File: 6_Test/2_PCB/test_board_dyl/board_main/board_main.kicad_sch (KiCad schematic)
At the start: 26 parts, among them J1 GND_Plane_Jumpers, J2 Analog_Inputs, J3 IOVDD_Jumpers, J4 Digital_Discovery_Output, J5 Power_Input, J6 Clock_Input

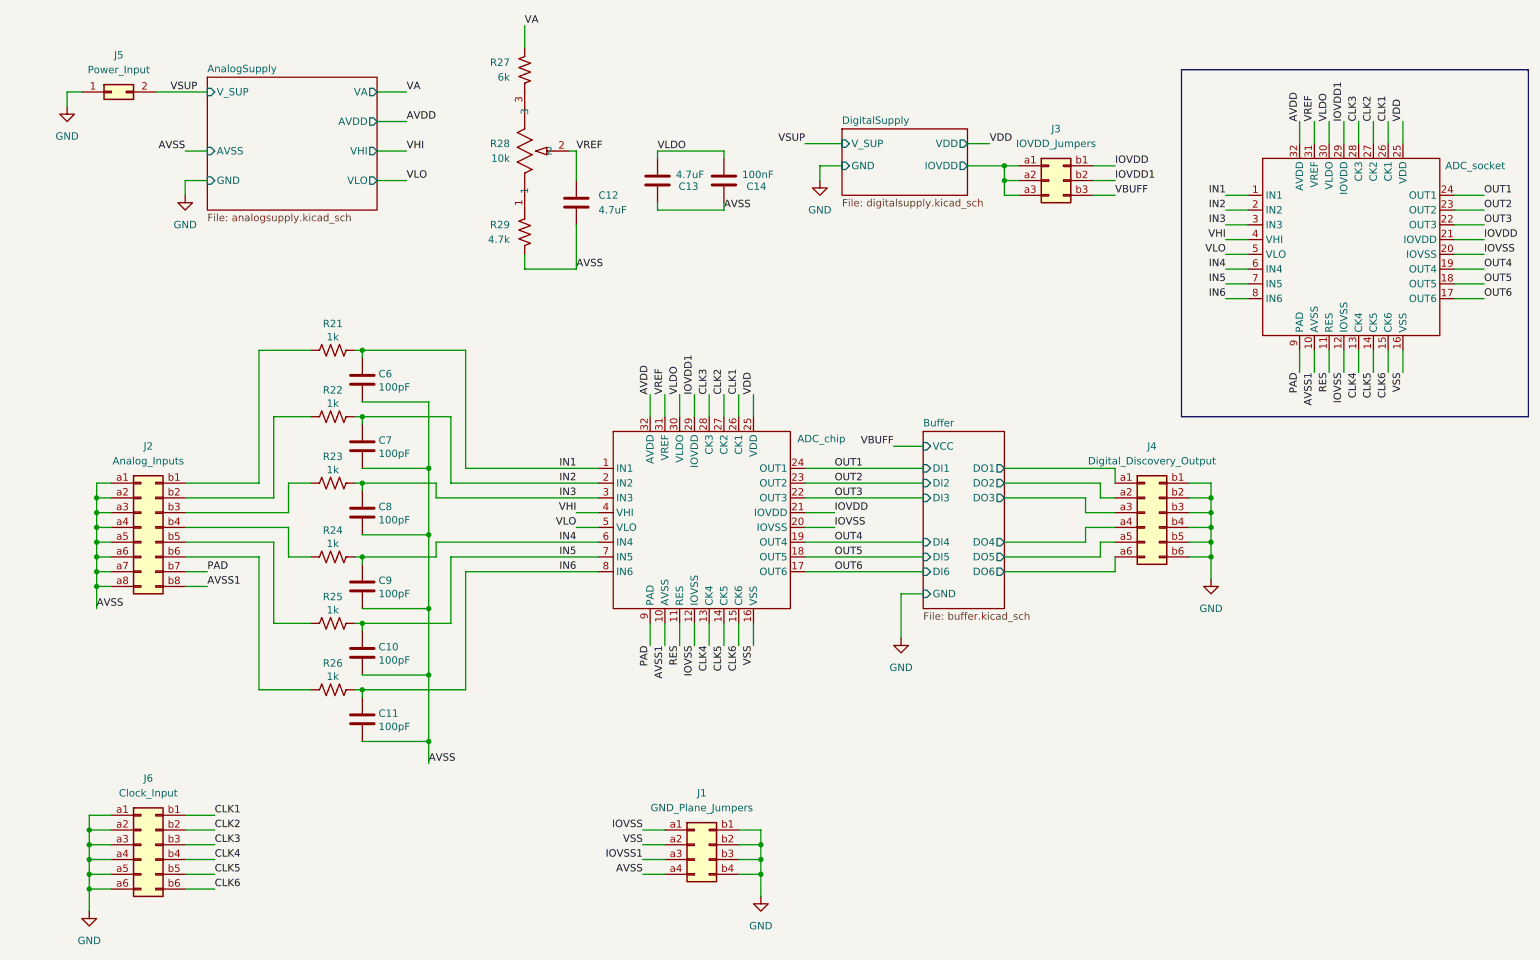
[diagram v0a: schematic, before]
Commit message: Fixed comments
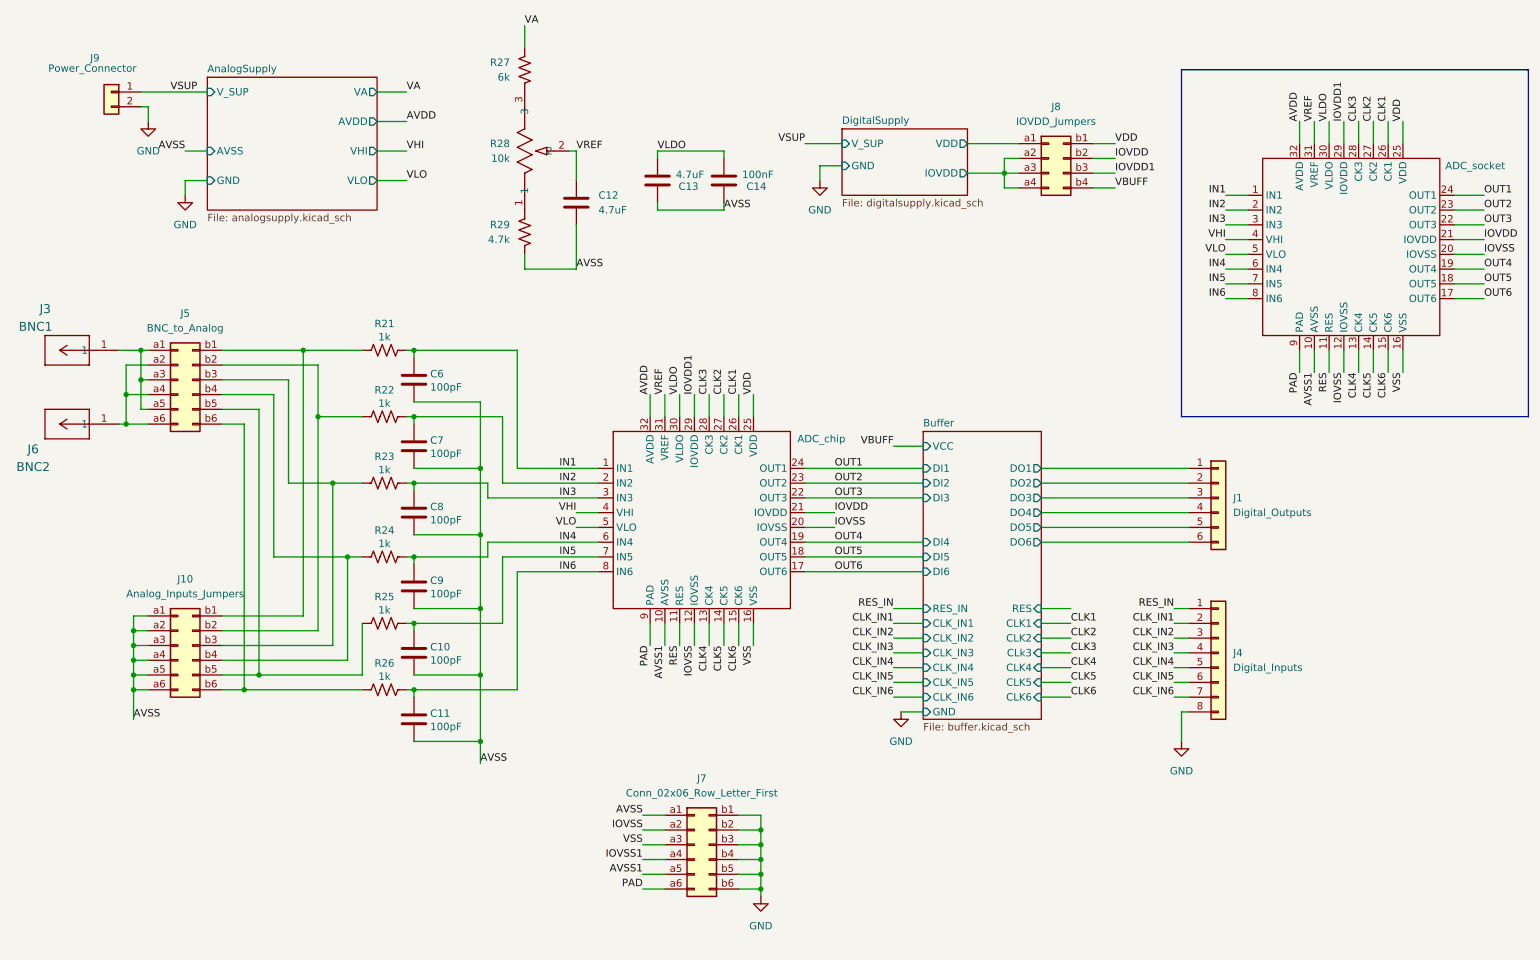
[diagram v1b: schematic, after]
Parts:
- removed J1: GND_Plane_Jumpers, Connector_PinHeader_2.54mm:PinHeader_2x04_P2.54mm_Vertical, symbol Connector_Generic:Conn_02x04_Row_Letter_First
- removed J2: Analog_Inputs, symbol Connector_Generic:Conn_02x08_Row_Letter_First
- removed J3: IOVDD_Jumpers, symbol Connector_Generic:Conn_02x03_Row_Letter_First
- removed J4: Digital_Discovery_Output, symbol Connector_Generic:Conn_02x06_Row_Letter_First
- removed J5: Power_Input, symbol Connector_Generic:Conn_02x01
- removed J6: Clock_Input, symbol Connector_Generic:Conn_02x06_Row_Letter_First
- added J1: Digital_Outputs, symbol Connector_Generic:Conn_01x06
- added J10: Analog_Inputs_Jumpers, symbol Connector_Generic:Conn_02x06_Row_Letter_First
- added J3: BNC1, CONN_1274571-1_TYCO, symbol bnc_mini:1274571-1
- added J4: Digital_Inputs, symbol Connector_Generic:Conn_01x08
- added J5: BNC_to_Analog, symbol Connector_Generic:Conn_02x06_Row_Letter_First
- added J6: BNC2, CONN_1274571-1_TYCO, symbol bnc_mini:1274571-1
- added J7: Conn_02x06_Row_Letter_First, symbol Connector_Generic:Conn_02x06_Row_Letter_First
- added J8: IOVDD_Jumpers, symbol Connector_Generic:Conn_02x04_Row_Letter_First
- added J9: Power_Connector, symbol Connector_Generic:Conn_01x02
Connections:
- net AVSS: now also J10.a1 (Pin_a1), J10.a2 (Pin_a2), J10.a3 (Pin_a3), J10.a4 (Pin_a4), J10.a5 (Pin_a5), J10.a6 (Pin_a6), J7.a1 (Pin_a1)
- net AVSS1: now also J7.a5 (Pin_a5)
- net Buffer/DO1: now also J1.1 (Pin_1)
- net Buffer/DO2: now also J1.2 (Pin_2)
- net Buffer/DO3: now also J1.3 (Pin_3)
- net Buffer/DO4: now also J1.4 (Pin_4)
- net Buffer/DO5: now also J1.5 (Pin_5)
- net Buffer/DO6: now also J1.6 (Pin_6)
- net DigitalSupply/IOVDD: now also J8.a2 (Pin_a2), J8.a3 (Pin_a3), J8.a4 (Pin_a4)
- net GND: now also J4.8 (Pin_8), J7.b1 (Pin_b1), J7.b2 (Pin_b2), J7.b3 (Pin_b3), J7.b4 (Pin_b4), J7.b5 (Pin_b5), J7.b6 (Pin_b6), J9.2 (Pin_2)
- net IOVDD: now also J8.b2 (Pin_b2)
- net IOVDD1: now also J8.b3 (Pin_b3)
- net IOVSS: now also J7.a2 (Pin_a2)
- net IOVSS1: now also J7.a4 (Pin_a4)
- net PAD: now also J7.a6 (Pin_a6)
- net VBUFF: now also J8.b4 (Pin_b4)
- net VDD: now also J8.b1 (Pin_b1)
- net VSS: now also J7.a3 (Pin_a3)
- net VSUP: now also J9.1 (Pin_1)
- net at R24.1: now also J10.b4 (Pin_b4), J5.b4 (Pin_b4)
- net at R25.1: now also J10.b5 (Pin_b5), J5.b5 (Pin_b5)
- net at R23.1: now also J10.b3 (Pin_b3), J5.b3 (Pin_b3)
- net at R21.1: now also J10.b1 (Pin_b1), J5.b1 (Pin_b1)
- net at R22.1: now also J10.b2 (Pin_b2), J5.b2 (Pin_b2)
- net at R26.1: now also J10.b6 (Pin_b6), J5.b6 (Pin_b6)
- new net: J5.a2 (Pin_a2), J5.a4 (Pin_a4), J5.a6 (Pin_a6), J6.1
- new net: J3.1, J5.a1 (Pin_a1), J5.a3 (Pin_a3), J5.a5 (Pin_a5)
- new net CLK_IN1: J4.2 (Pin_2)
- new net CLK_IN2: J4.3 (Pin_3)
- new net CLK_IN3: J4.4 (Pin_4)
- new net CLK_IN4: J4.5 (Pin_5)
- new net CLK_IN5: J4.6 (Pin_6)
- new net CLK_IN6: J4.7 (Pin_7)
- new net DigitalSupply/VDD: J8.a1 (Pin_a1)
- new net RES_IN: J4.1 (Pin_1)
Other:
- sheet Buffer ports: added CLK1, CLK2, CLK4, CLK5, CLK6, CLK_IN1, CLK_IN2, CLK_IN3, CLK_IN4, CLK_IN5, CLK_IN6, CLk3, RES, RES_IN; removed none
- moved on the sheet: C10, C11, C6, C7, C8, C9, R21, R22, R23, R24, R25, R26

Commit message: final draft of board done.
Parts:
- J10: footprint (none) -> Connector_PinHeader_1.00mm:PinHeader_1x15_P1.00mm_Vertical
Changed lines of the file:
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@@
 			)
 		)
-		(property "Footprint" ""
+		(property "Footprint" "Connector_PinHeader_1.00mm:PinHeader_1x15_P1.00mm_Vertical"
 			(at 44.45 135.89 0)
 			(effects
